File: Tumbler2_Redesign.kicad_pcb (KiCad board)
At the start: 2 copper layers, 77 x 84 mm, 114 parts, among them J1 Conn_01x02, J2 Conn_01x05, J3 Conn_01x10, J4 Conn_01x10, J5 USB_C_Receptacle_USB2.0_16P, J6 USB_C_Receptacle_USB2.0_16P, J7 Conn_01x04, J8 Conn_01x06, J9 Conn_01x06, Q1 MMBT3904, Q3 MMBT3904, SW1 SW_Push, SW2 SW_Push, SW3 SW_Push, U1 CH340C, U11 TB6612FNG, U12 AMS1117-5.0, U2 LSM6DSV, U3 AP63203WU, U4 ESP32-S3-WROOM-1, U8 USBLC6-2SC6, U9 USBLC6-2SC6

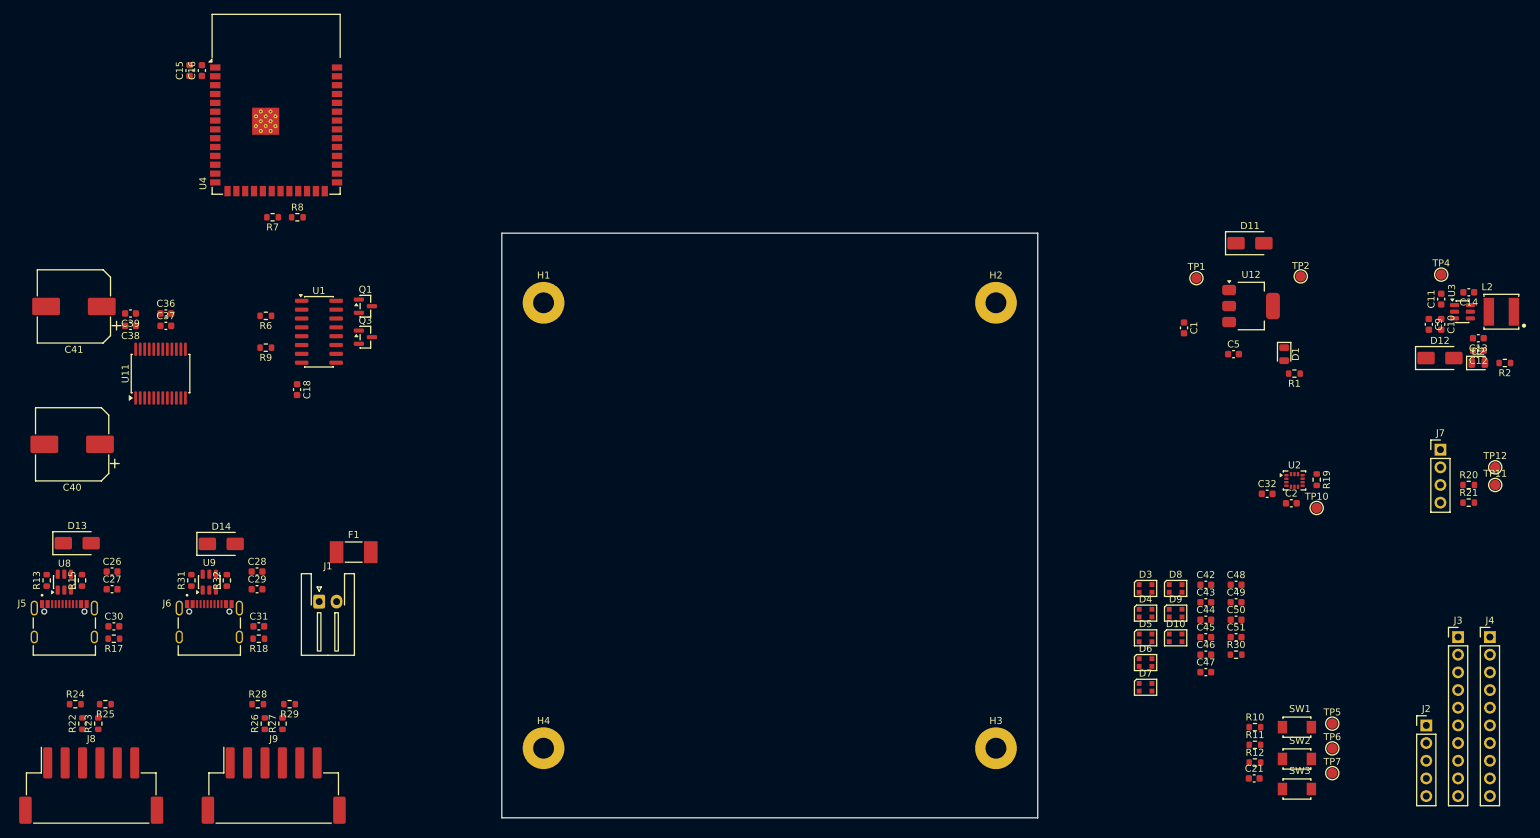
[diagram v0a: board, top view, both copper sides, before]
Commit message: Sketch out component placement
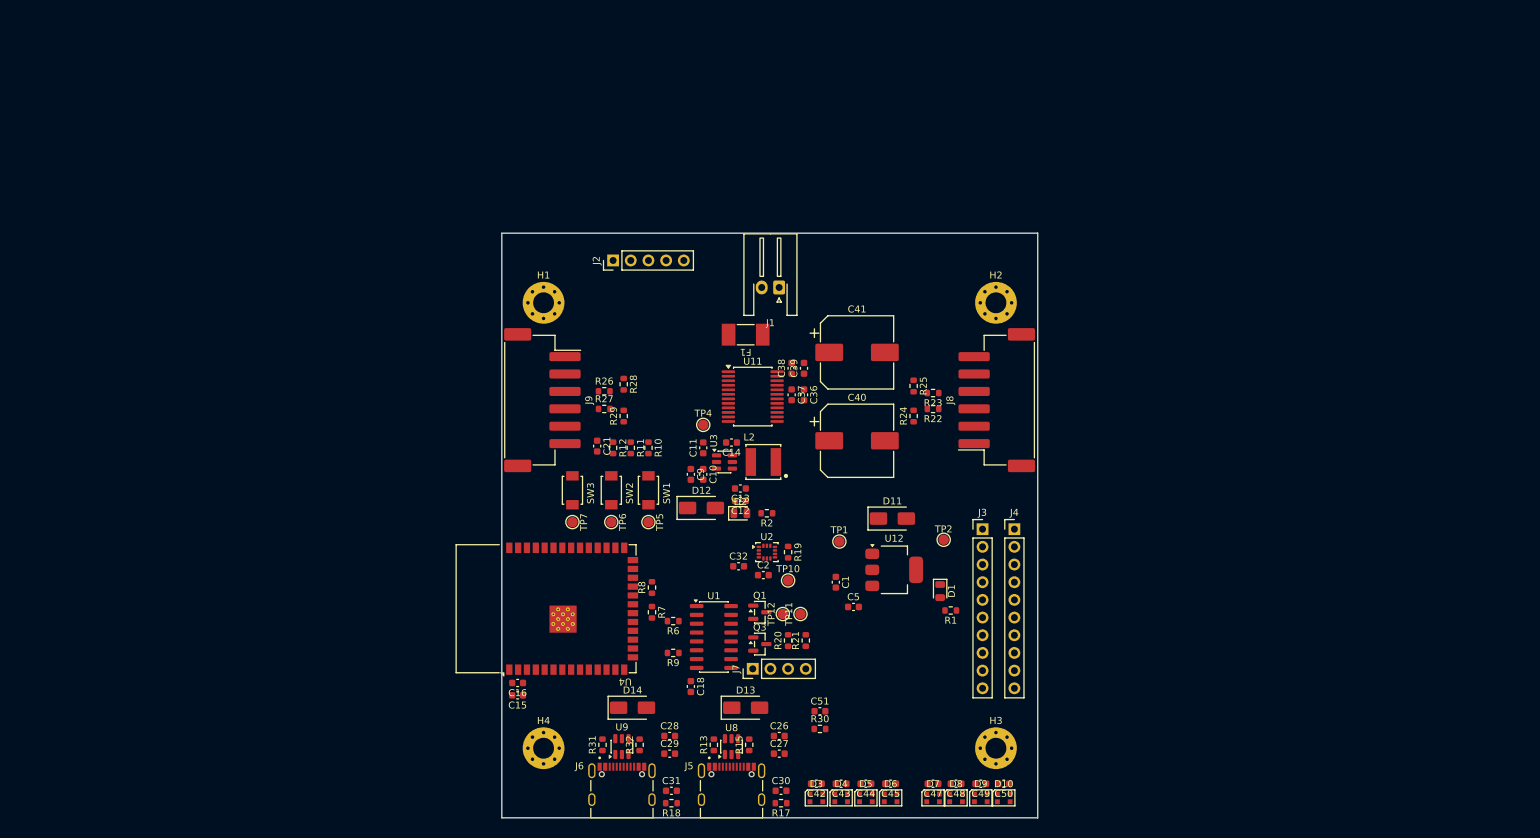
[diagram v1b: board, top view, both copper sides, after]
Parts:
- removed C46: 10uF, Capacitor_SMD:C_0603_1608Metric
- H1, H2, H3, H4: footprint MountingHole:MountingHole_3mm_Pad -> MountingHole:MountingHole_3mm_Pad_Via
- moved J8 141.4 mm to (184.9, 85.3), turned to 90 degrees
- moved J2 134.6 mm to (129.8, 65.3), turned to 90 degrees
- moved R22 130.3 mm to (175.8, 86.6), turned to 180 degrees
- moved R23 129.0 mm to (175.8, 84.3), turned to 180 degrees
- moved R24 127.4 mm to (173.0, 87.6), turned to 90 degrees
- moved R25 124.8 mm to (173.0, 83.3), turned to -90 degrees
- moved TP7 115.0 mm to (124.0, 102.9), turned to -90 degrees
- moved C40 112.8 mm to (164.8, 91.2), turned to 0 degrees
- moved C41 112.7 mm to (164.8, 78.5), turned to 0 degrees
- moved SW3 112.6 mm to (124.0, 98.3), turned to -90 degrees
- moved TP6 108.6 mm to (129.5, 102.9), turned to -90 degrees
- moved D12 108.3 mm to (142.5, 100.8)
- moved L2 108.2 mm to (151.4, 94.2)
- moved C12 108.2 mm to (148.1, 99.8)
- moved C13 108.2 mm to (148.1, 98.0)
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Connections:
- net /MCU/INT renamed /MCU/INT1
